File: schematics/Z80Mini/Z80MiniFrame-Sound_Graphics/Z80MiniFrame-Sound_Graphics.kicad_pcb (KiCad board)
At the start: 2 copper layers, 194.3 x 105.4 mm, 70 parts, among them J1 Conn_02x20_Odd_Even, J2 RGB Out, J3 Conn_01x03_Male, U1 TMS9929A, U12 74LS32, U13 74LS139, U14 TL084, U2 74LS574, U3 74LS574, U4 74LS574, U5 AS6C62256-55PCN, U6 74HC04, U7 AY-3-8910, U8 74LS02, U9 LM386, X1 ACO-2MHz, Y1 Crystal

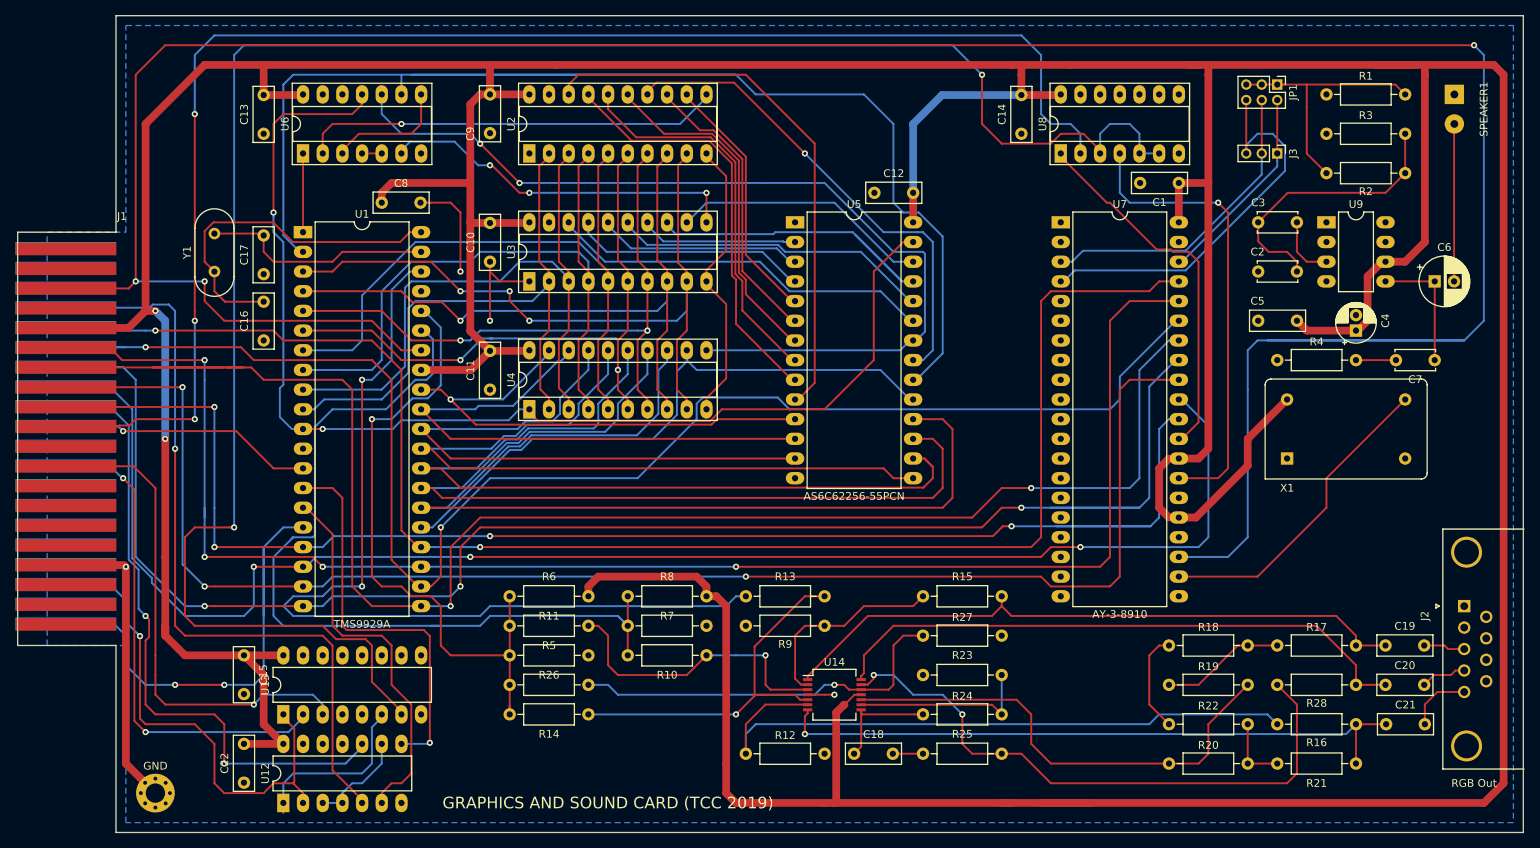
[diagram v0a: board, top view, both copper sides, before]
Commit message: Latest modifications
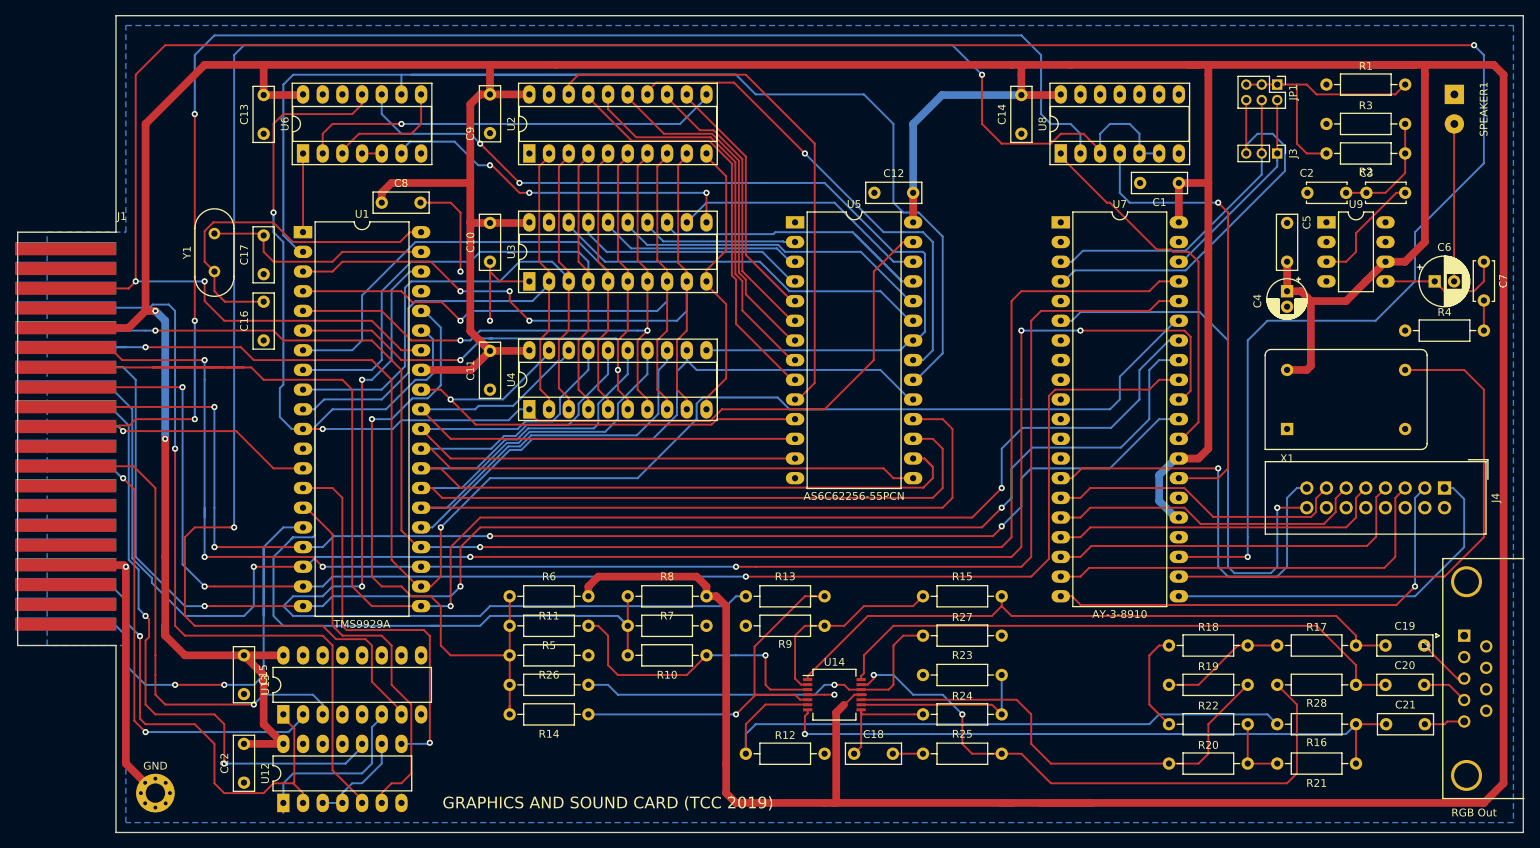
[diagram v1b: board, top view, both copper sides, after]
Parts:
- added J4: IO_PORT, Connector_IDC:IDC-Header_2x08_P2.54mm_Vertical, F.Cu at (229.9, 102.9)
- moved R4 16.9 mm to (224.8, 82.5)
- moved C3 14.5 mm to (224.8, 64.8)
- moved C7 14.2 mm to (234.9, 73.7), turned to 270 degrees
- moved C2 12.0 mm to (217.2, 64.8)
- moved C4 10.2 mm to (209.6, 77.5), turned to 270 degrees
- moved C5 7.73 mm to (209.6, 73.7), turned to 90 degrees
- moved J2 3.81 mm to (232.4, 121.9)
- moved X1 3.81 mm to (209.6, 95.2)
- moved R2 2.54 mm to (224.8, 59.7)
- moved R1 1.27 mm to (214.6, 50.8)
- moved R3 1.27 mm to (214.6, 55.9)
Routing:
- net Net-(J4-Pad16): track 0.00 -> 71.2 mm, vias 0 -> 1
- net Net-(J4-Pad3): track 0.00 -> 60.8 mm, vias 0 -> 1
- net Net-(J4-Pad15): track 0.00 -> 55.4 mm, vias 0 -> 1
- net Net-(J4-Pad5): track 0.00 -> 54.0 mm
- net Net-(J4-Pad1): track 0.00 -> 48.8 mm
- net Net-(J4-Pad7): track 0.00 -> 48.6 mm
- net Net-(J4-Pad9): track 0.00 -> 43.5 mm
- net Net-(J4-Pad11): track 0.00 -> 41.6 mm
- net Net-(J4-Pad13): track 0.00 -> 39.3 mm
- net /graphicsProcessor/RESET: track 380.0 -> 348.7 mm, vias 3 -> 4
- net Net-(U7-Pad22): track 40.9 -> 71.7 mm
- net Net-(C2-Pad1): track 36.5 -> 15.0 mm
- net /D7: track 187.5 -> 172.2 mm
- net /D6: track 198.1 -> 213.4 mm, vias 3 -> 4
- net /D4: track 205.8 -> 192.3 mm
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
